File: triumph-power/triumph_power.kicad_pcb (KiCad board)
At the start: 2 copper layers, 53.3 x 33 mm, 22 parts, among them J1 JST_XH_vert_01x04, J2 JST_XH_vert_01x04, U1 RS-1212D

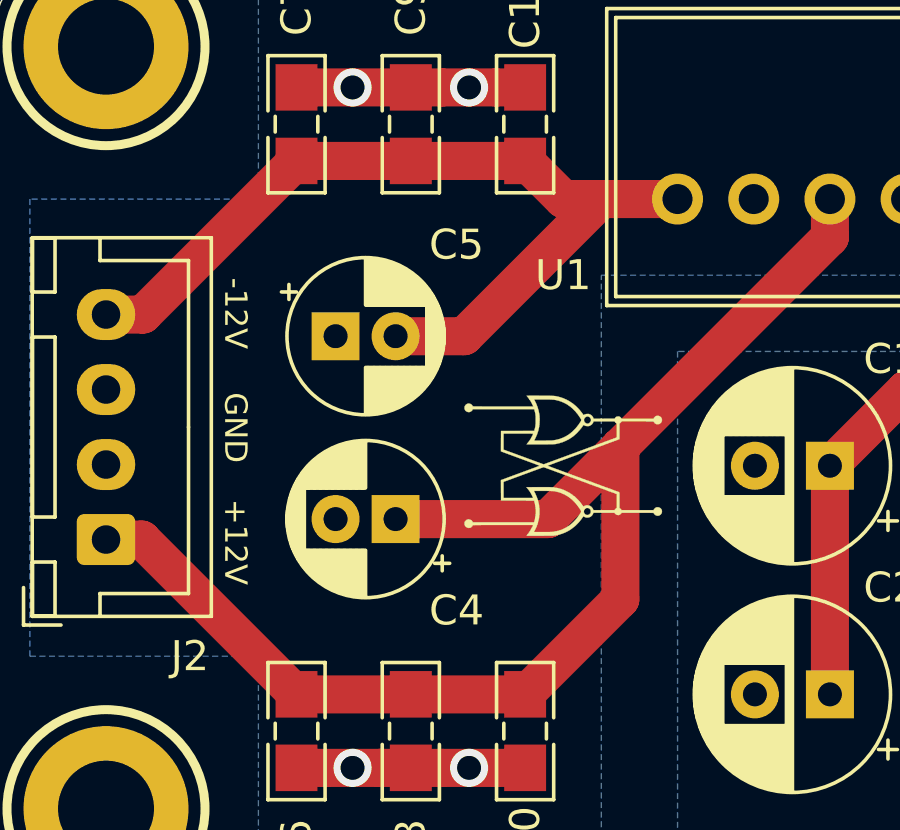
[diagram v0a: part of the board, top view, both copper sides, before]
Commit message: Generate gerbers
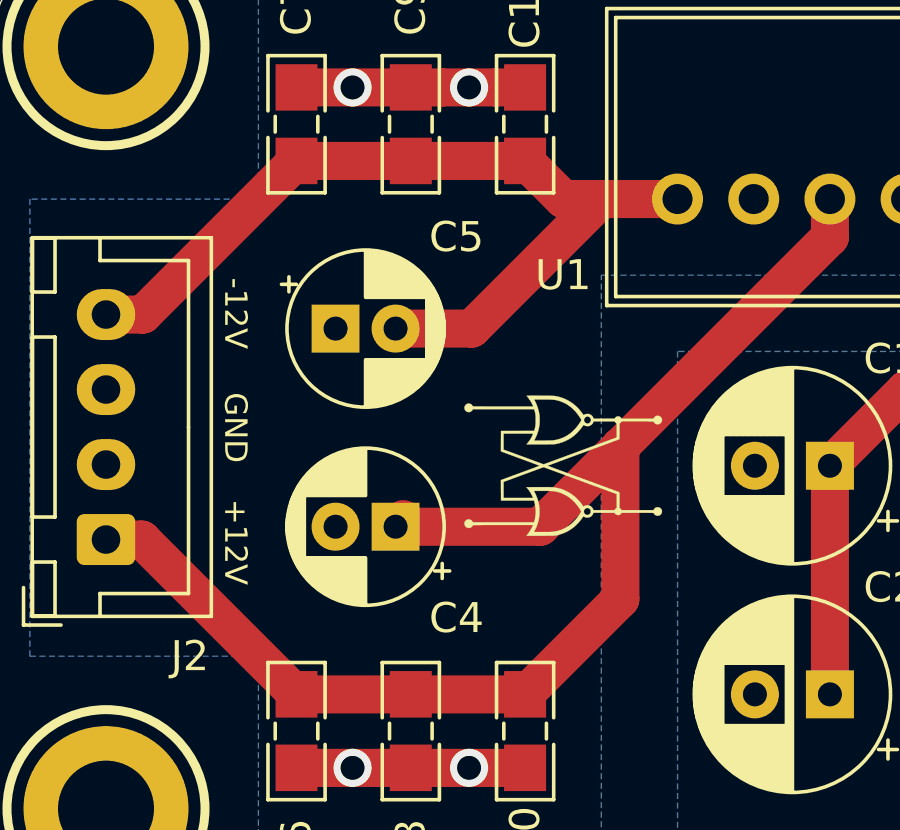
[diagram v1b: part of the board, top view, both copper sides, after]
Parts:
- moved C4 0.25 mm to (136.7, 112.5)
- moved C5 0.25 mm to (134.7, 105.9)
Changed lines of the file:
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@@
     (thickness 1.6)
     (drawings 23)
-    (tracks 61)
+    (tracks 63)
     (zones 0)
     (modules 22)
@@
     (solder_mask_min_width 0.25)
     (aux_axis_origin 0 0)
+    (grid_origin 123.19 125.73)
     (visible_elements 7FFFFFFF)
     (pcbplotparams
@@
   )
   (module Capacitor_THT:CP_Radial_D5.0mm_P2.00mm (layer F.Cu)
-    (at 134.652 106.172)
+    (at 134.652 105.918)
     (descr "CP, Radial series, Radial, pin pitch=2.00mm, , diameter=5mm, Electrolytic Capacitor")
     (tags "CP Radial series Radial pin pitch 2.00mm  diameter 5mm Electrolytic Capacitor")
@@
   )
   (module Capacitor_THT:CP_Radial_D5.0mm_P2.00mm (layer F.Cu)
-    (at 136.652 112.268 180)
+    (at 136.652 112.522 180)
     (descr "CP, Radial series, Radial, pin pitch=2.00mm, , diameter=5mm, Electrolytic Capacitor")
     (tags "CP Radial series Radial pin pitch 2.00mm  diameter 5mm Electrolytic Capacitor")
@@
   (segment (start 137.16 118.11) (end 140.97 118.11) (width 1.27) (layer F.Cu) (net 4))
   (segment (start 151.13 101.6) (end 151.13 102.87) (width 1.27) (layer F.Cu) (net 4))
-  (segment (start 141.732 112.268) (end 136.652 112.268) (width 1.27) (layer F.Cu) (net 4))
   (segment (start 144.145 109.855) (end 144.145 114.935) (width 1.27) (layer F.Cu) (net 4))
   (segment (start 151.13 102.87) (end 144.145 109.855) (width 1.27) (layer F.Cu) (net 4))
+  (segment (start 144.145 114.935) (end 140.97 118.11) (width 1.27) (layer F.Cu) (net 4))
+  (segment (start 136.906 112.268) (end 136.652 112.522) (width 1.27) (layer F.Cu) (net 4))
   (segment (start 144.145 109.855) (end 141.732 112.268) (width 1.27) (layer F.Cu) (net 4))
-  (segment (start 144.145 114.935) (end 140.97 118.11) (width 1.27) (layer F.Cu) (net 4))
-  (segment (start 138.938 106.172) (end 136.652 106.172) (width 1.27) (layer F.Cu) (net 5))
+  (segment (start 141.478 112.522) (end 141.732 112.268) (width 1.27) (layer F.Cu) (net 4))
+  (segment (start 136.652 112.522) (end 141.478 112.522) (width 1.27) (layer F.Cu) (net 4))
   (segment (start 146.05 101.6) (end 143.51 101.6) (width 1.27) (layer F.Cu) (net 5))
-  (segment (start 143.51 101.6) (end 138.938 106.172) (width 1.27) (layer F.Cu) (net 5))
   (segment (start 140.97 100.33) (end 142.24 101.6) (width 1.27) (layer F.Cu) (net 5))
   (segment (start 142.24 101.6) (end 143.51 101.6) (width 1.27) (layer F.Cu) (net 5))
@@
   (segment (start 128.23 105.45) (end 133.35 100.33) (width 1.27) (layer F.Cu) (net 5))
   (segment (start 127 105.45) (end 128.23 105.45) (width 1.27) (layer F.Cu) (net 5))
+  (segment (start 139.192 105.918) (end 136.652 105.918) (width 1.27) (layer F.Cu) (net 5))
+  (segment (start 143.51 101.6) (end 139.192 105.918) (width 1.27) (layer F.Cu) (net 5))
   (segment (start 166.37 114.3) (end 162.56 114.3) (width 1.27) (layer F.Cu) (net 6))
   (segment (start 167.68 112.99) (end 166.37 114.3) (width 1.27) (layer F.Cu) (net 6))
